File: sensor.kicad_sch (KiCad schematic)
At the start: 17 parts, among them Q1 SI2301CDS-T1-GE3, U4 ST_SENSOR_2, U5 IIS3DHHCTR

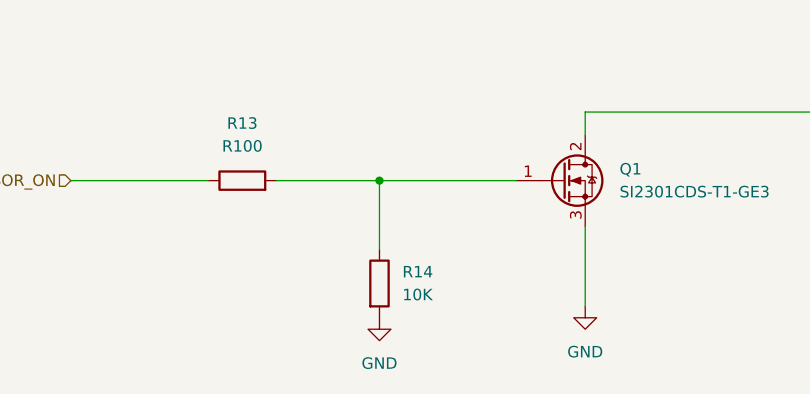
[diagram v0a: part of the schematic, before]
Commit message: remove hellen
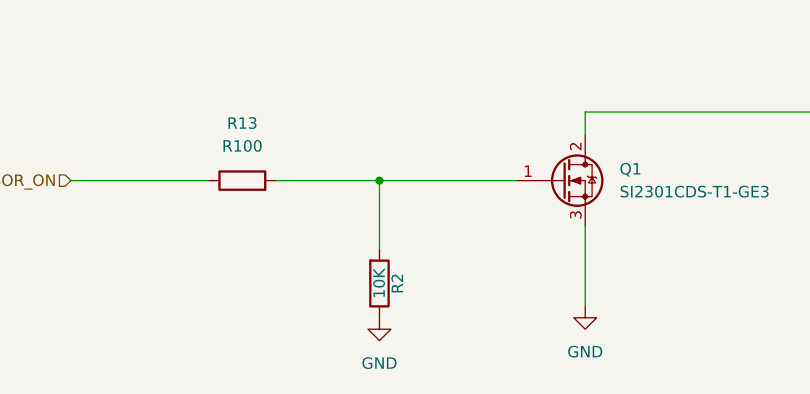
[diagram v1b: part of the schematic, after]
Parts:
- removed R14: 10K, symbol Device:R
- added R2: 10K, Resistor_SMD:R_0603_1608Metric, symbol Device:R
- U5: footprint IIS3DHHCTR:IC_IIS3DHHCTR -> dnt:CCLGA-16L_5X5X1P7_STM
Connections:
- net GND: now also R2.1
- net at Q1.1 (G), R13.2: now also R2.2
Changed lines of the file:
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@@
+	(symbol
+		(lib_id "Device:R")
+		(at 73.66 128.27 0)
+		(mirror x)
+		(unit 1)
+		(exclude_from_sim no)
+		(in_bom yes)
+		(on_board yes)
+		(dnp no)
+		(property "Reference" "R2"
+			(at 75.692 128.27 90)
+			(effects
+				(font
+					(size 1.27 1.27)
+				)
+			)
+		)
+		(property "Value" "10K"
+			(at 73.66 128.27 90)
+			(effects
+				(font
+					(size 1.27 1.27)
+				)
+			)
+		)
+		(property "Footprint" "Resistor_SMD:R_0603_1608Metric"
+			(at 132.842 186.69 90)
+			(effects
+				(font
+					(size 1.524 1.524)
+				)
+				(hide yes)
+			)
+		)
+		(property "Datasheet" "~"
+			(at 222.25 187.325 0)
+			(effects
+				(font
+					(size 1.524 1.524)
+				)
+				(hide yes)
+			)
+		)
+		(property "Description" "Resistor"
+			(at 73.66 128.27 0)
+			(effects
+				(font
+					(size 1.27 1.27)
+				)
+				(hide yes)
+			)
+		)
+		(property "Part #" "RMCF0603JT10K0"
+			(at -29.21 30.48 0)
+			(effects
+				(font
+					(size 1.27 1.27)
+				)
+				(hide yes)
+			)
+		)
+		(property "VEND" "DIGI"
+			(at -29.21 30.48 0)
+			(effects
+				(font
+					(size 1.27 1.27)
+				)
+				(hide yes)
+			)
+		)
+		(property "VEND#" "RMCF0603JT10K0CT-ND"
+			(at -29.21 30.48 0)
+			(effects
+				(font
+					(size 1.27 1.27)
+				)
+				(hide yes)
+			)
+		)
+		(property "Manufacturer" "StackPole"
+			(at -29.21 30.48 0)
+			(effects
+				(font
+					(size 1.27 1.27)
+				)
+				(hide yes)
+			)
+		)
+		(property "LCSC" "C25804"
+			(at 73.66 128.27 0)
+			(effects
+				(font
+					(size 1.27 1.27)
+				)
+				(hide yes)
+			)
+		)
+		(pin "1"
+		)
+		(pin "2"
+		)
+		(instances
+			(project "l8-kicad"
+				(path "/8d063f79-9282-4820-bcf4-1ff3c006cf08/801ffdec-7184-42a0-bbdb-64e97598ca97"
+					(reference "R2")
+					(unit 1)
+				)
+			)
+		)
+	)
 	(symbol
 		(lib_id "Device:R")
@@
 	)
 	(symbol
-		(lib_id "Device:R")
-		(at 73.66 128.27 0)
-		(unit 1)
-		(exclude_from_sim no)
-		(in_bom yes)
-		(on_board yes)
-		(dnp no)
-		(fields_autoplaced yes)
-		(property "Reference" "R14"
-			(at 76.2 126.9999 0)
-			(effects
-				(font
-					(size 1.27 1.27)
-				)
-				(justify left)
-			)
-		)
-		(property "Value" "10K"
-			(at 76.2 129.5399 0)
-			(effects
-				(font
-					(size 1.27 1.27)
-				)
-				(justify left)
-			)
-		)
-		(property "Footprint" ""
-			(at 71.882 128.27 90)
-			(effects
-				(font
-					(size 1.27 1.27)
-				)
-				(hide yes)
-			)
-		)
-		(property "Datasheet" "~"
-			(at 73.66 128.27 0)
-			(effects
-				(font
-					(size 1.27 1.27)
-				)
-				(hide yes)
-			)
-		)
-		(property "Description" "Resistor"
-			(at 73.66 128.27 0)
-			(effects
-				(font
-					(size 1.27 1.27)
-				)
-				(hide yes)
-			)
-		)
-		(pin "1"
-		)
-		(pin "2"
-		)
-		(instances
-			(project ""
-				(path "/8d063f79-9282-4820-bcf4-1ff3c006cf08/801ffdec-7184-42a0-bbdb-64e97598ca97"
-					(reference "R14")
-					(unit 1)
-				)
-			)
-		)
-	)
-	(symbol
 		(lib_id "l8-kicad-rescue:GND-power")
 		(at 73.66 132.08 0)
@@
 			)
 		)
-		(property "Footprint" "IIS3DHHCTR:IC_IIS3DHHCTR"
+		(property "Footprint" "dnt:CCLGA-16L_5X5X1P7_STM"
 			(at 92.71 59.69 0)
 			(effects
